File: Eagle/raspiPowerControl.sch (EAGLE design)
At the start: 10 parts, among them Q1 FDN360P, T1 BC847

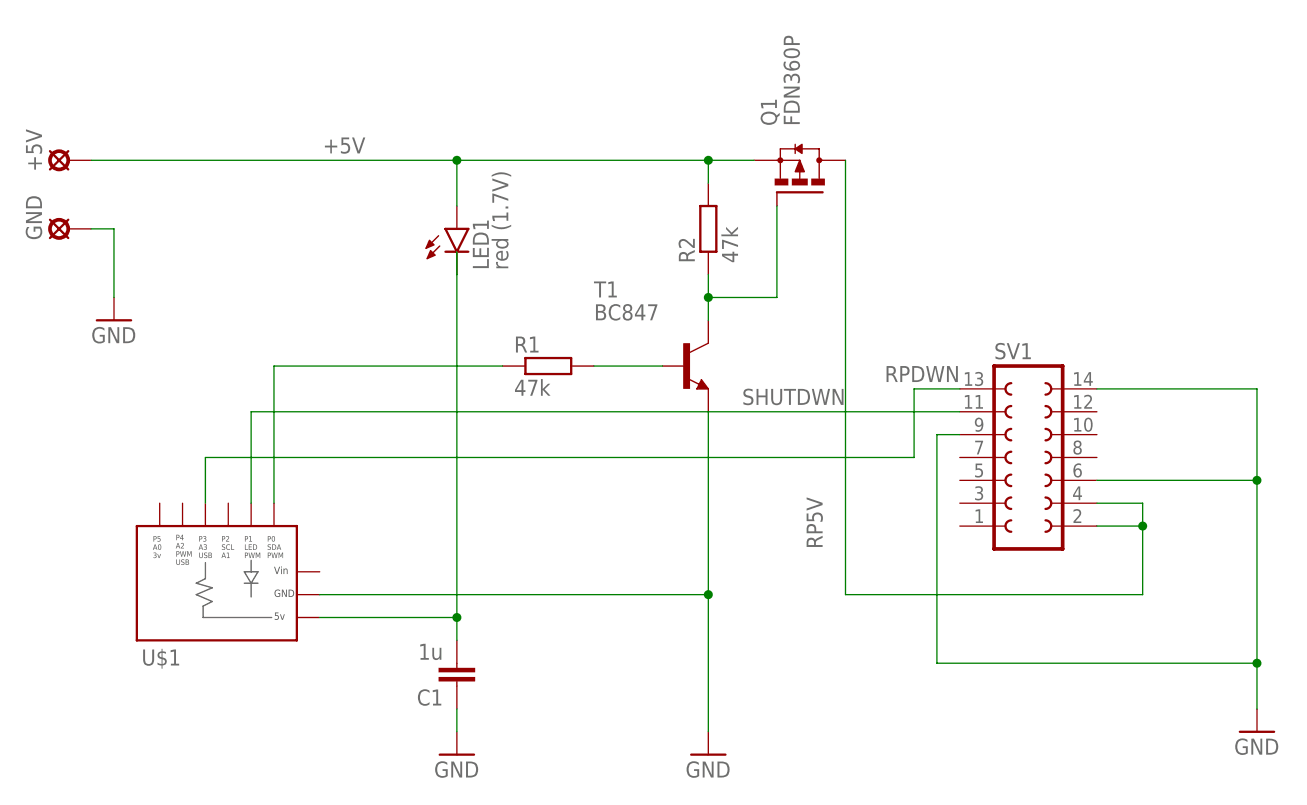
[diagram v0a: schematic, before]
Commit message: Update Eagle
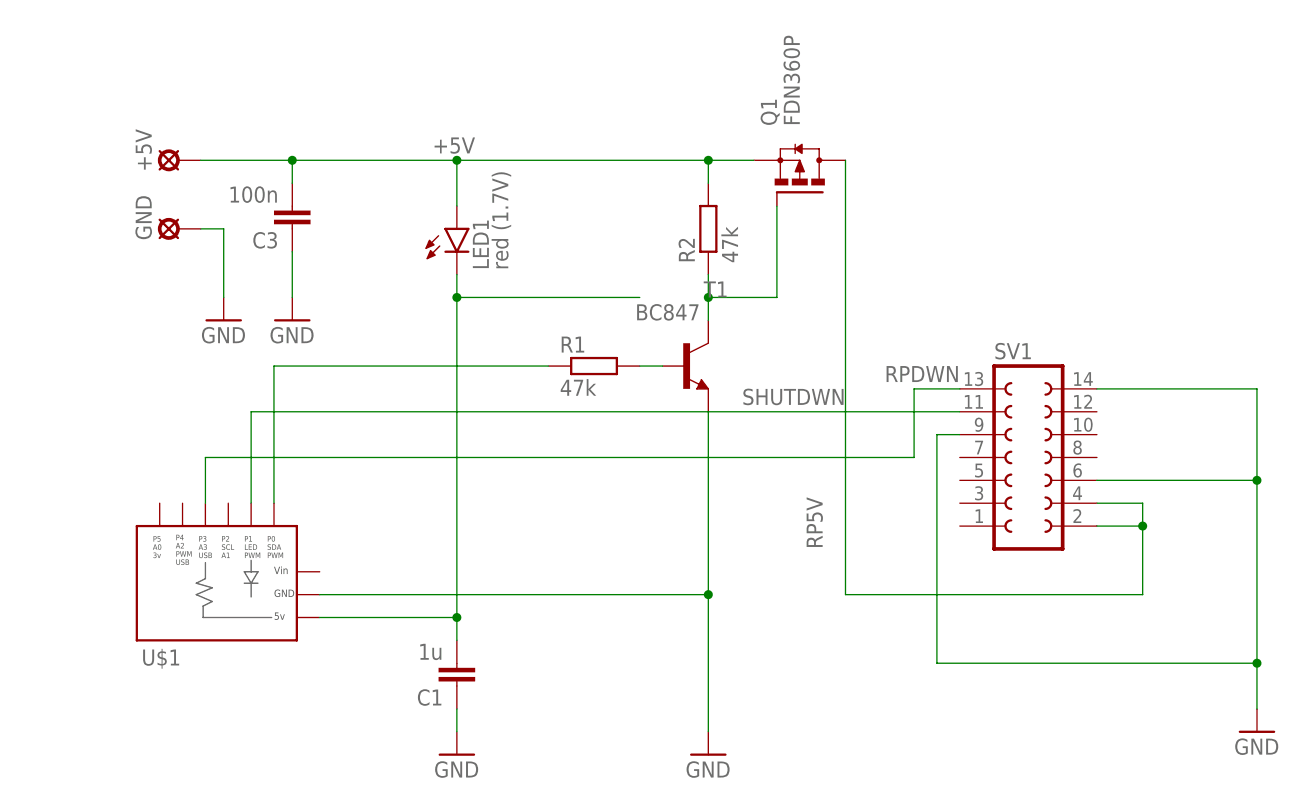
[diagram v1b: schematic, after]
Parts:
- added C3: 100n, rcl:C-EUC0805
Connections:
- net +5V: now also C3.2
- net GND: now also C3.1
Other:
- moved on the sheet: +5V, GND, R1
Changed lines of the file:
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@@
 <part name="C1" library="rcl" library_urn="urn:adsk.eagle:library:334" deviceset="C-EU" device="C0805" package3d_urn="urn:adsk.eagle:package:23617/2" value="1u"/>
 <part name="GND4" library="supply1" library_urn="urn:adsk.eagle:library:371" deviceset="GND" device=""/>
+<part name="C3" library="rcl" library_urn="urn:adsk.eagle:library:334" deviceset="C-EU" device="C0805" package3d_urn="urn:adsk.eagle:package:23617/2" value="100n"/>
+<part name="GND5" library="supply1" library_urn="urn:adsk.eagle:library:371" deviceset="GND" device=""/>
 </parts>
 <sheets>
@@
 </instance>
 <instance part="T1" gate="G$1" x="60.96" y="48.26" smashed="yes">
-<attribute name="NAME" x="50.8" y="55.88" size="1.778" layer="95"/>
-<attribute name="VALUE" x="50.8" y="53.34" size="1.778" layer="96"/>
+<attribute name="NAME" x="62.992" y="55.88" size="1.778" layer="95"/>
+<attribute name="VALUE" x="55.372" y="53.34" size="1.778" layer="96"/>
 </instance>
 <instance part="Q1" gate="G$1" x="73.66" y="68.58" smashed="yes" rot="R90">
@@
 <attribute name="VALUE" x="121.92" y="5.08" size="1.778" layer="96"/>
 </instance>
-<instance part="R1" gate="G$1" x="45.72" y="48.26" smashed="yes">
-<attribute name="NAME" x="41.91" y="49.7586" size="1.778" layer="95"/>
-<attribute name="VALUE" x="41.91" y="44.958" size="1.778" layer="96"/>
+<instance part="R1" gate="G$1" x="50.8" y="48.26" smashed="yes">
+<attribute name="NAME" x="46.99" y="49.7586" size="1.778" layer="95"/>
+<attribute name="VALUE" x="46.99" y="44.958" size="1.778" layer="96"/>
 </instance>
 <instance part="R2" gate="G$1" x="63.5" y="63.5" smashed="yes" rot="R90">
@@
 <attribute name="VALUE" x="60.96" y="2.54" size="1.778" layer="96"/>
 </instance>
-<instance part="+5V" gate="1" x="-7.62" y="71.12" smashed="yes" rot="R90">
-<attribute name="NAME" x="-10.541" y="69.85" size="1.778" layer="95" rot="R90"/>
+<instance part="+5V" gate="1" x="4.572" y="71.12" smashed="yes" rot="R90">
+<attribute name="NAME" x="1.651" y="69.85" size="1.778" layer="95" rot="R90"/>
 </instance>
-<instance part="GND" gate="1" x="-7.62" y="63.5" smashed="yes" rot="R90">
-<attribute name="NAME" x="-10.541" y="62.23" size="1.778" layer="95" rot="R90"/>
+<instance part="GND" gate="1" x="4.572" y="63.5" smashed="yes" rot="R90">
+<attribute name="NAME" x="1.651" y="62.23" size="1.778" layer="95" rot="R90"/>
 </instance>
-<instance part="GND3" gate="1" x="-2.54" y="53.34" smashed="yes">
-<attribute name="VALUE" x="-5.08" y="50.8" size="1.778" layer="96"/>
+<instance part="GND3" gate="1" x="9.652" y="53.34" smashed="yes">
+<attribute name="VALUE" x="7.112" y="50.8" size="1.778" layer="96"/>
 </instance>
 <instance part="LED1" gate="G$1" x="35.56" y="63.5" smashed="yes">
@@
 <instance part="GND4" gate="1" x="35.56" y="5.08" smashed="yes">
 <attribute name="VALUE" x="33.02" y="2.54" size="1.778" layer="96"/>
+</instance>
+<instance part="C3" gate="G$1" x="17.272" y="63.5" smashed="yes" rot="R180">
+<attribute name="NAME" x="15.748" y="63.119" size="1.778" layer="95" rot="R180"/>
+<attribute name="VALUE" x="15.748" y="68.199" size="1.778" layer="96" rot="R180"/>
+</instance>
+<instance part="GND5" gate="1" x="17.272" y="53.34" smashed="yes">
+<attribute name="VALUE" x="14.732" y="50.8" size="1.778" layer="96"/>
 </instance>
 </instances>
@@
 <pinref part="GND" gate="1" pin="MP"/>
 <pinref part="GND3" gate="1" pin="GND"/>
-<wire x1="-5.08" y1="63.5" x2="-2.54" y2="63.5" width="0.1524" layer="91"/>
-<wire x1="-2.54" y1="63.5" x2="-2.54" y2="55.88" width="0.1524" layer="91"/>
+<wire x1="7.112" y1="63.5" x2="9.652" y2="63.5" width="0.1524" layer="91"/>
+<wire x1="9.652" y1="63.5" x2="9.652" y2="55.88" width="0.1524" layer="91"/>
 </segment>
 <segment>
@@
 <pinref part="C1" gate="G$1" pin="1"/>
 <wire x1="35.56" y1="7.62" x2="35.56" y2="10.16" width="0.1524" layer="91"/>
+</segment>
+<segment>
+<pinref part="C3" gate="G$1" pin="1"/>
+<pinref part="GND5" gate="1" pin="GND"/>
+<wire x1="17.272" y1="60.96" x2="17.272" y2="55.88" width="0.1524" layer="91"/>
 </segment>
 </net>
@@
 <wire x1="63.5" y1="71.12" x2="68.58" y2="71.12" width="0.1524" layer="91"/>
 <pinref part="+5V" gate="1" pin="MP"/>
-<wire x1="-5.08" y1="71.12" x2="35.56" y2="71.12" width="0.1524" layer="91"/>
 <junction x="63.5" y="71.12"/>
+<label x="37.592" y="73.66" size="1.778" layer="95" rot="R180"/>
+<wire x1="7.112" y1="71.12" x2="17.272" y2="71.12" width="0.1524" layer="91"/>
+<wire x1="17.272" y1="71.12" x2="35.56" y2="71.12" width="0.1524" layer="91"/>
+<pinref part="C3" gate="G$1" pin="2"/>
+<wire x1="35.56" y1="71.12" x2="63.5" y2="71.12" width="0.1524" layer="91"/>
+<wire x1="17.272" y1="71.12" x2="17.272" y2="68.58" width="0.1524" layer="91"/>
+<junction x="17.272" y="71.12"/>
 <pinref part="LED1" gate="G$1" pin="A"/>
-<wire x1="35.56" y1="71.12" x2="63.5" y2="71.12" width="0.1524" layer="91"/>
 <wire x1="35.56" y1="66.04" x2="35.56" y2="71.12" width="0.1524" layer="91"/>
 <junction x="35.56" y="71.12"/>
-<label x="25.4" y="73.66" size="1.778" layer="95" rot="R180"/>
 </segment>
 </net>
@@
 <pinref part="R1" gate="G$1" pin="2"/>
 <pinref part="T1" gate="G$1" pin="B"/>
-<wire x1="50.8" y1="48.26" x2="58.42" y2="48.26" width="0.1524" layer="91"/>
+<wire x1="55.88" y1="48.26" x2="58.42" y2="48.26" width="0.1524" layer="91"/>
 </segment>
 </net>
@@
 <pinref part="R1" gate="G$1" pin="1"/>
 <wire x1="15.24" y1="33.02" x2="15.24" y2="48.26" width="0.1524" layer="91"/>
-<wire x1="15.24" y1="48.26" x2="40.64" y2="48.26" width="0.1524" layer="91"/>
+<wire x1="15.24" y1="48.26" x2="45.72" y2="48.26" width="0.1524" layer="91"/>
 </segment>
 </net>
 <net name="PWR" class="0">
 <segment>
-<pinref part="LED1" gate="G$1" pin="C"/>
-<wire x1="35.56" y1="58.42" x2="35.56" y2="60.96" width="0.1524" layer="91"/>
-<wire x1="35.56" y1="58.42" x2="35.56" y2="20.32" width="0.1524" layer="91"/>
 <pinref part="U$1" gate="G$1" pin="5V"/>
 <wire x1="35.56" y1="20.32" x2="20.32" y2="20.32" width="0.1524" layer="91"/>
 <pinref part="C1" gate="G$1" pin="2"/>
 <wire x1="35.56" y1="17.78" x2="35.56" y2="20.32" width="0.1524" layer="91"/>
+<wire x1="35.56" y1="55.88" x2="35.56" y2="20.32" width="0.1524" layer="91"/>
 <junction x="35.56" y="20.32"/>
+<wire x1="35.56" y1="55.88" x2="55.88" y2="55.88" width="0.1524" layer="91"/>
+<pinref part="LED1" gate="G$1" pin="C"/>
+<wire x1="35.56" y1="55.88" x2="35.56" y2="58.42" width="0.1524" layer="91"/>
+<junction x="35.56" y="55.88"/>
 </segment>
 </net>
